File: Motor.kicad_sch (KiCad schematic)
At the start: 6 parts

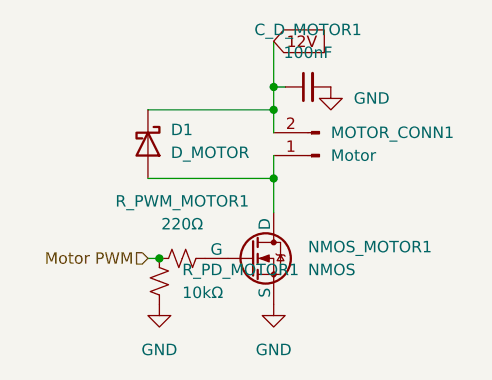
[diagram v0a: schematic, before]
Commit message: Checkpoint
Checkpoint, pre battery telemetry, pre new stm
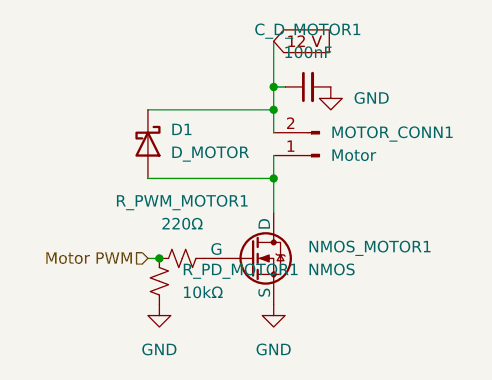
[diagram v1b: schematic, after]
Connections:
- net 12V renamed 12 V
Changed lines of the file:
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@@
 		)
 	)
-	(global_label "12V"
+	(global_label "12 V"
 		(shape input)
 		(at 40.64 22.86 0)
@@
 		)
 		(property "Intersheetrefs" "${INTERSHEET_REFS}"
-			(at 47.1328 22.86 0)
+			(at 48.1004 22.86 0)
 			(hide yes)
 			(show_name no)
